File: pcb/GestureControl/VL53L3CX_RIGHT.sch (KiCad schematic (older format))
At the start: 14 parts, among them U10 VL53L3CXV0DH_RIGHT, U4 VL53L3CXV0DH_RIGHT, U8 VL53L3CXV0DH_RIGHT

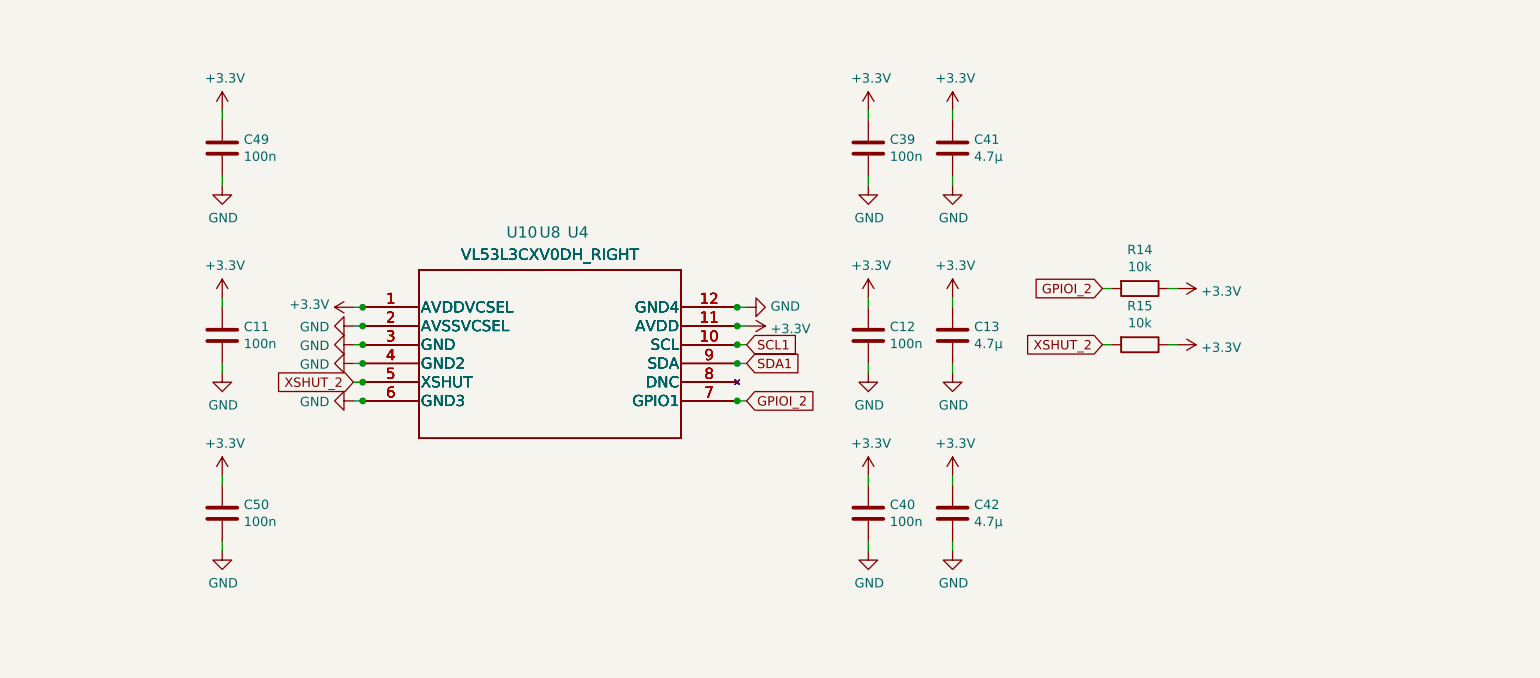
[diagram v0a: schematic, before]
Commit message: add PCBV0.11
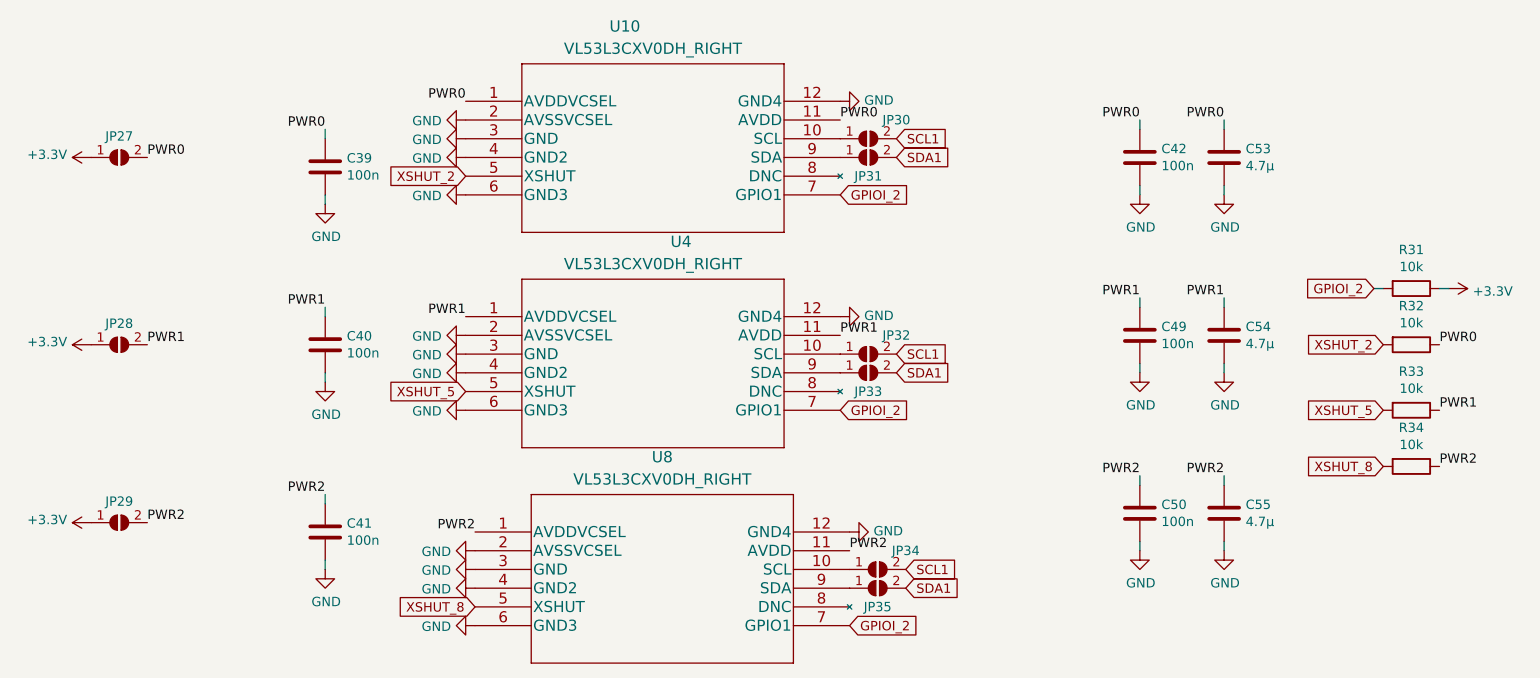
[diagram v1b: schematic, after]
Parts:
- removed C11, C12: 100n, Capacitor_SMD:C_0603_1608Metric_Pad1.08x0.95mm_HandSolder, symbol Device:C
- removed C13: 4.7µ, Capacitor_SMD:C_0805_2012Metric_Pad1.18x1.45mm_HandSolder, symbol Device:C
- removed R14, R15: 10k, Resistor_SMD:R_0805_2012Metric_Pad1.20x1.40mm_HandSolder, symbol Device:R
- added C53, C54, C55: 4.7µ, Capacitor_SMD:C_0805_2012Metric_Pad1.18x1.45mm_HandSolder, symbol Device:C
- added JP27, JP28, JP29, JP30, JP31, JP32, JP33, JP34, JP35: SolderJumper_2_Open, Jumper:SolderJumper-2_P1.3mm_Open_Pad1.0x1.5mm, symbol Jumper:SolderJumper_2_Open
- added R31, R32, R33, R34: 10k, Resistor_SMD:R_0805_2012Metric_Pad1.20x1.40mm_HandSolder, symbol Device:R
- C41, C42: value 4.7µ -> 100n; footprint Capacitor_SMD:C_0805_2012Metric_Pad1.18x1.45mm_HandSolder -> Capacitor_SMD:C_0603_1608Metric_Pad1.08x0.95mm_HandSolder
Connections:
- net +3V3: now also JP27.1 (A), JP28.1 (A), JP29.1 (A), R31.1; no longer C39.1, C40.1, C41.1, C42.1, C49.1, C50.1, U10.1 (AVDDVCSEL), U10.11 (AVDD), U4.1 (AVDDVCSEL), U4.11 (AVDD), U8.1 (AVDDVCSEL), U8.11 (AVDD)
- net GND: now also C53.2, C54.2, C55.2
- net GPIOI_2: now also R31.2
- net SCL1: now also JP30.2 (B), JP32.2 (B), JP34.2 (B); no longer U10.10 (SCL), U4.10 (SCL), U8.10 (SCL)
- net SDA1: now also JP31.2 (B), JP33.2 (B), JP35.2 (B); no longer U10.9 (SDA), U4.9 (SDA), U8.9 (SDA)
- net XSHUT_2: now also R32.2; no longer U4.5 (XSHUT), U8.5 (XSHUT)
- new net: JP34.1 (A), U8.10 (SCL)
- new net: JP35.1 (A), U8.9 (SDA)
- new net: JP30.1 (A), U10.10 (SCL)
- new net: JP31.1 (A), U10.9 (SDA)
- new net: JP32.1 (A), U4.10 (SCL)
- new net: JP33.1 (A), U4.9 (SDA)
- new net PWR0: C39.1, C42.1, C53.1, JP27.2 (B), R32.1, U10.1 (AVDDVCSEL), U10.11 (AVDD)
- new net PWR1: C40.1, C49.1, C54.1, JP28.2 (B), R33.1, U4.1 (AVDDVCSEL), U4.11 (AVDD)
- new net PWR2: C41.1, C50.1, C55.1, JP29.2 (B), R34.1, U8.1 (AVDDVCSEL), U8.11 (AVDD)
- new net XSHUT_5: R33.2, U4.5 (XSHUT)
- new net XSHUT_8: R34.2, U8.5 (XSHUT)
- now unconnected: U10.8 (DNC), U4.8 (DNC), U8.8 (DNC)
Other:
- moved on the sheet: U10, U4, U8
